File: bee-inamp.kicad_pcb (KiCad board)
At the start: 2 copper layers, 13.7 x 53.3 mm, 12 parts, among them J1 Conn_01x02_Male, J2 Conn_01x02_Male, J3 Conn_01x02_Male, J4 Conn_01x02_Male

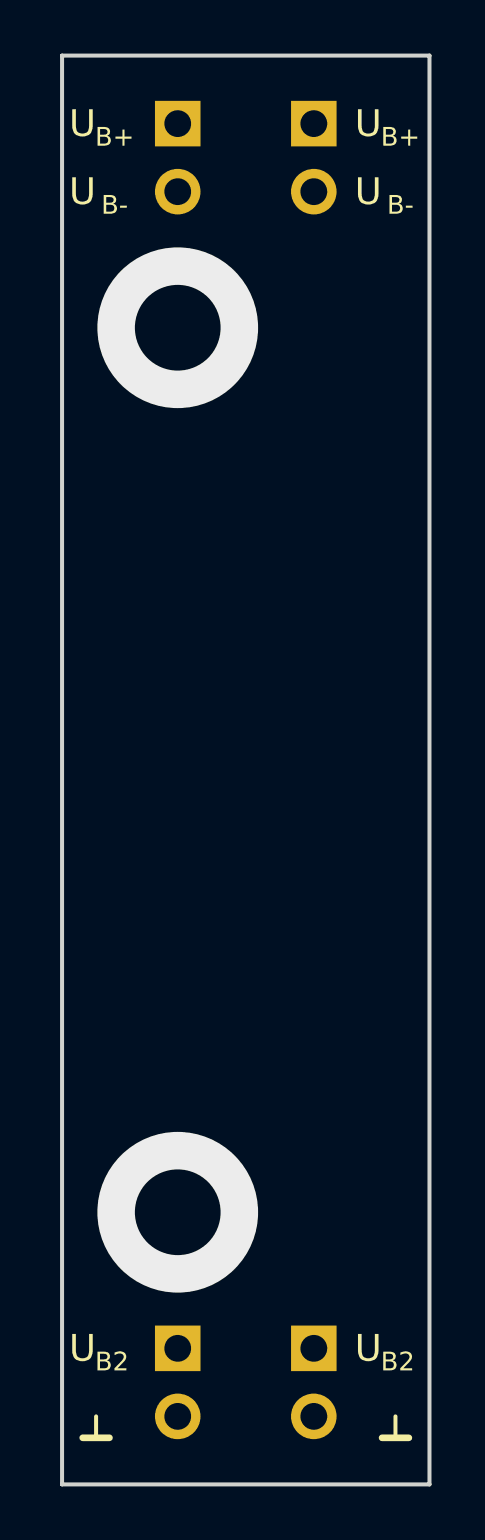
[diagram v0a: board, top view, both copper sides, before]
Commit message: schematic and layout
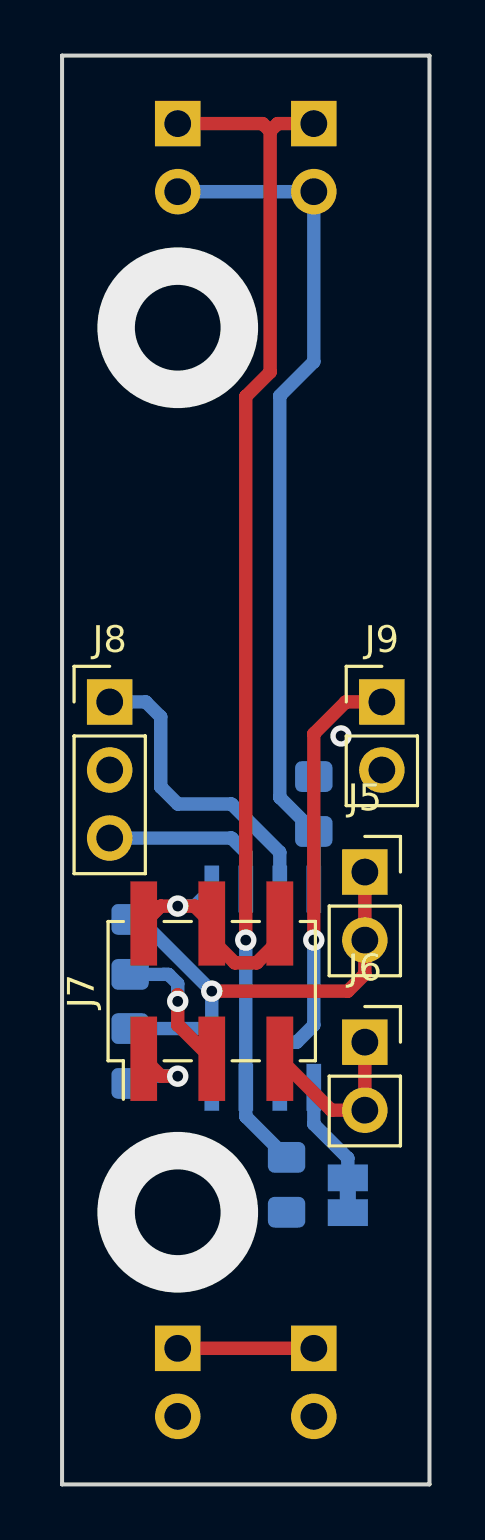
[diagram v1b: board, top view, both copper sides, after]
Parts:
- removed REF** (x2): Text_U_B+_Silkscreen, Symbol-emt:Text_U_B+_Silkscreen
- removed REF** (x2): Text_U_B-_Silkscreen, Symbol-emt:Text_U_B-_Silkscreen
- removed REF** (x2): Text_U_B2_Silkscreen, Symbol-emt:Text_U_B2_Silkscreen
- removed REF** (x2): Symbol_GND_Silkscreen, Symbol-emt:Symbol_GND_Silkscreen
- added C1: 0.1µF, Capacitor_SMD:C_0805_2012Metric_Pad1.15x1.40mm_HandSolder, B.Cu at (82.8, 131.1)
- added C2: 0.1µF, Capacitor_SMD:C_0805_2012Metric_Pad1.15x1.40mm_HandSolder, B.Cu at (83.8, 116.8)
- added J5: Conn_01x02, Connector_PinSocket_2.54mm:PinSocket_1x02_P2.54mm_Vertical, F.Cu at (85.7, 119.4)
- added J6: Conn_01x02, Connector_PinSocket_2.54mm:PinSocket_1x02_P2.54mm_Vertical, F.Cu at (85.7, 125.7)
- added J7: Conn_02x03_Odd_Even, Connector_PinHeader_2.54mm:PinHeader_2x03_P2.54mm_Vertical_SMD, F.Cu at (80.0, 123.8)
- added J8: Conn_01x03, Connector_PinHeader_2.54mm:PinHeader_1x03_P2.54mm_Vertical, F.Cu at (76.2, 113.0)
- added J9: Conn_01x02, Connector_PinHeader_2.54mm:PinHeader_1x02_P2.54mm_Vertical, F.Cu at (86.4, 113.0)
- added JP1: SolderJumper_2_Bridged, Jumper:SolderJumper-2_P1.3mm_Bridged_Pad1.0x1.5mm, B.Cu at (85.1, 131.4)
- added R1: 16k, Resistor_SMD:R_0805_2012Metric_Pad1.15x1.40mm_HandSolder, B.Cu at (77.0, 126.2)
- added R2: 820R, Resistor_SMD:R_0805_2012Metric_Pad1.15x1.40mm_HandSolder, B.Cu at (77.0, 122.2)
- added U1: INA126, Package_SO:SO-8_5.3x6.2mm_P1.27mm, B.Cu at (81.9, 123.7)
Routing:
- net +15V: track 0.00 -> 44.6 mm, vias 0 -> 1
- net -15V: track 0.00 -> 32.2 mm
- net Rg_2: track 0.00 -> 20.6 mm, vias 0 -> 1
- net Net-(J9-Pad1): track 0.00 -> 16.9 mm, vias 0 -> 1
- net in+: track 0.00 -> 11.6 mm
- net Rg_1: track 0.00 -> 9.11 mm, vias 0 -> 1
- net in-: track 0.00 -> 6.67 mm
- net Net-(J6-Pad1): track 0.00 -> 6.51 mm
- net Net-(J7-Pad3): track 0.00 -> 5.52 mm, vias 0 -> 1
- net +5V: track 0.00 -> 5.08 mm
- net Net-(JP1-Pad1): track 0.00 -> 3.91 mm
- net Net-(J7-Pad1): track 0.00 -> 2.81 mm, vias 0 -> 1
- net GND: vias 0 -> 1
- added copper zone on B.Cu, net GND
- added copper zone on F.Cu, net GND
